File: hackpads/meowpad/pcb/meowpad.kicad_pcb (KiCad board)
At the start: 2 copper layers, 110 x 65.5 mm, 16 parts, among them J1 OLED_DISPLAY, SW1 SW_Push_45deg, SW2 SW_Push_45deg, SW3 SW_Push_45deg, SW4 SW_Push_45deg, SW6 SW_Push_45deg, U2 XIAO-RP2040-DIP

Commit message: oops i forgot to put xiao here
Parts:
- U2: value XIAO-RP2040-DIP -> XIAO HERE!!
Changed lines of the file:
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@@
 			)
 		)
-		(property "Value" "XIAO-RP2040-DIP"
+		(property "Value" "XIAO HERE!!"
 			(at 0 0 0)
 			(unlocked yes)

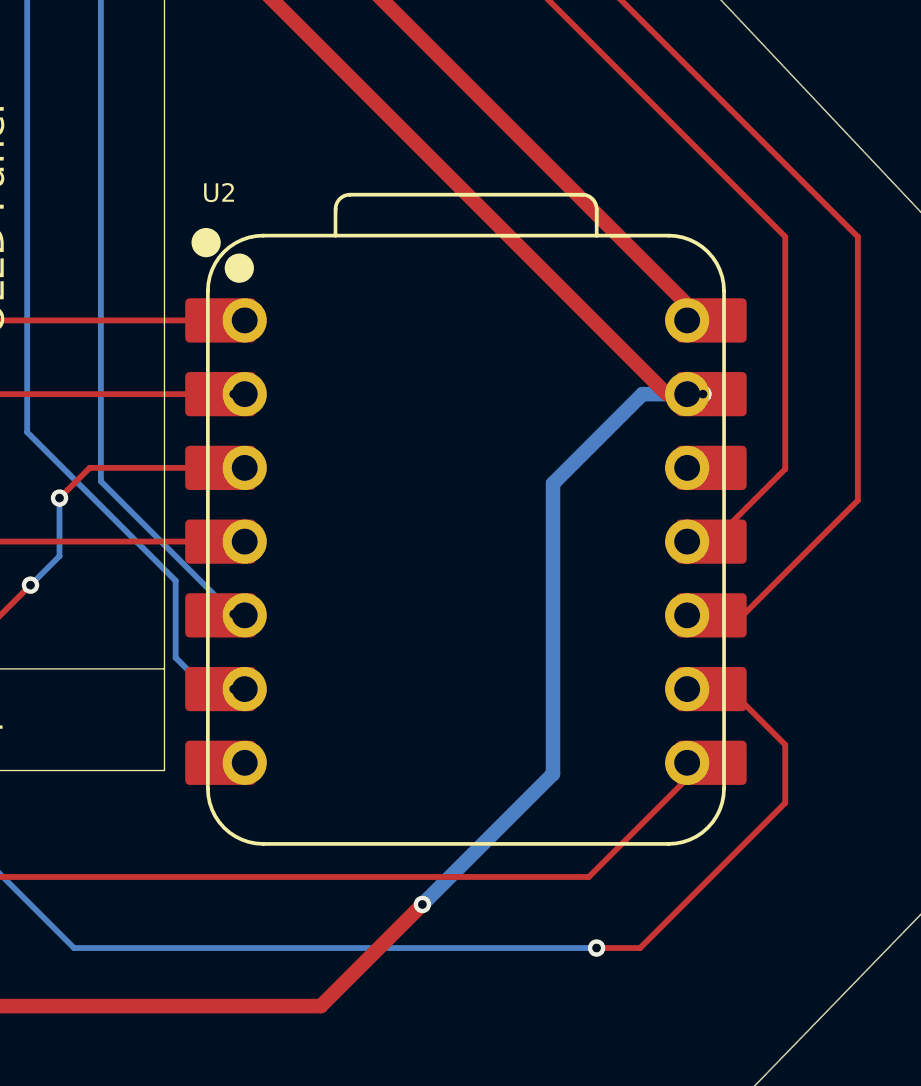
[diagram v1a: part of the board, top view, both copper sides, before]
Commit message: small edits
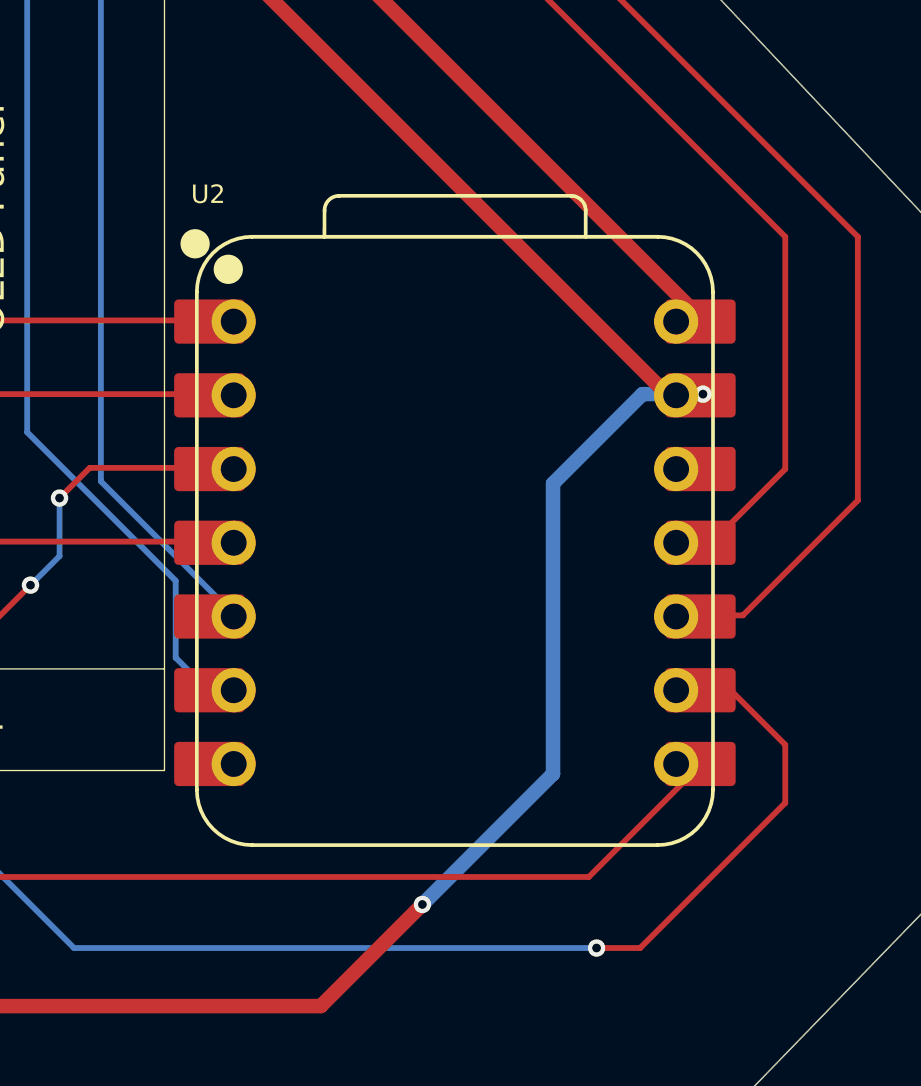
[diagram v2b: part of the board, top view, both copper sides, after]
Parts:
- moved U2 0.38 mm to (196.1, 100.5)
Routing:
- net GND: track 91.5 -> 89.5 mm
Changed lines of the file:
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@@
 	(footprint "Seeed Studio XIAO Series Library:XIAO-RP2040-DIP"
 		(layer "F.Cu")
-		(at 196.5 100.5)
+		(at 196.12 100.54)
 		(property "Reference" "U2"
 			(at -8.5 -12 0)
@@
 	)
 	(segment
-		(start 204.665 95.42)
-		(end 204.665 95.665)
-		(width 0.5)
-		(layer "F.Cu")
-		(net 1)
-	)
-	(segment
 		(start 191.5 116.5)
 		(end 195 113)
@@
 	)
 	(segment
-		(start 204.42 95.42)
-		(end 204.665 95.42)
-		(width 0.5)
-		(layer "F.Cu")
-		(net 1)
-	)
-	(segment
 		(start 189.5 81.5)
 		(end 203.42 95.42)
@@
 	)
 	(segment
-		(start 204.665 95.665)
-		(end 204.42 95.42)
-		(width 0.5)
-		(layer "F.Cu")
-		(net 1)
-	)
-	(segment
 		(start 185.92 81.5)
 		(end 189.5 81.5)
@@
 		(end 177 116.5)
 		(width 0.5)
-		(layer "F.Cu")
-		(net 1)
-	)
-	(segment
-		(start 203.42 95.42)
-		(end 204.665 95.42)
-		(width 0.2)
 		(layer "F.Cu")
 		(net 1)
@@
 	)
 	(segment
+		(start 202.58 95.42)
+		(end 199.5 98.5)
+		(width 0.5)
+		(layer "B.Cu")
+		(net 1)
+	)
+	(segment
+		(start 204.665 95.42)
+		(end 202.58 95.42)
+		(width 0.5)
+		(layer "B.Cu")
+		(net 1)
+	)
+	(segment
 		(start 199.5 98.5)
-		(end 202.58 95.42)
-		(width 0.5)
-		(layer "B.Cu")
-		(net 1)
-	)
-	(segment
-		(start 202.58 95.42)
-		(end 204.665 95.42)
-		(width 0.5)
-		(layer "B.Cu")
-		(net 1)
-	)
-	(segment
-		(start 199.5 108.5)
-		(end 199.5 98.5)
-		(width 0.5)
-		(layer "B.Cu")
-		(net 1)
-	)
-	(segment
-		(start 195 113)
 		(end 199.5 108.5)
 		(width 0.5)
@@
 		(layer "B.Cu")
 		(net 1)
+	)
+	(segment
+		(start 199.5 108.5)
+		(end 195 113)
+		(width 0.5)
+		(layer "B.Cu")
+		(net 1)
